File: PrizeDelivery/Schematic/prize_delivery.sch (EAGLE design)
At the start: 22 parts, among them Q1 IRL540

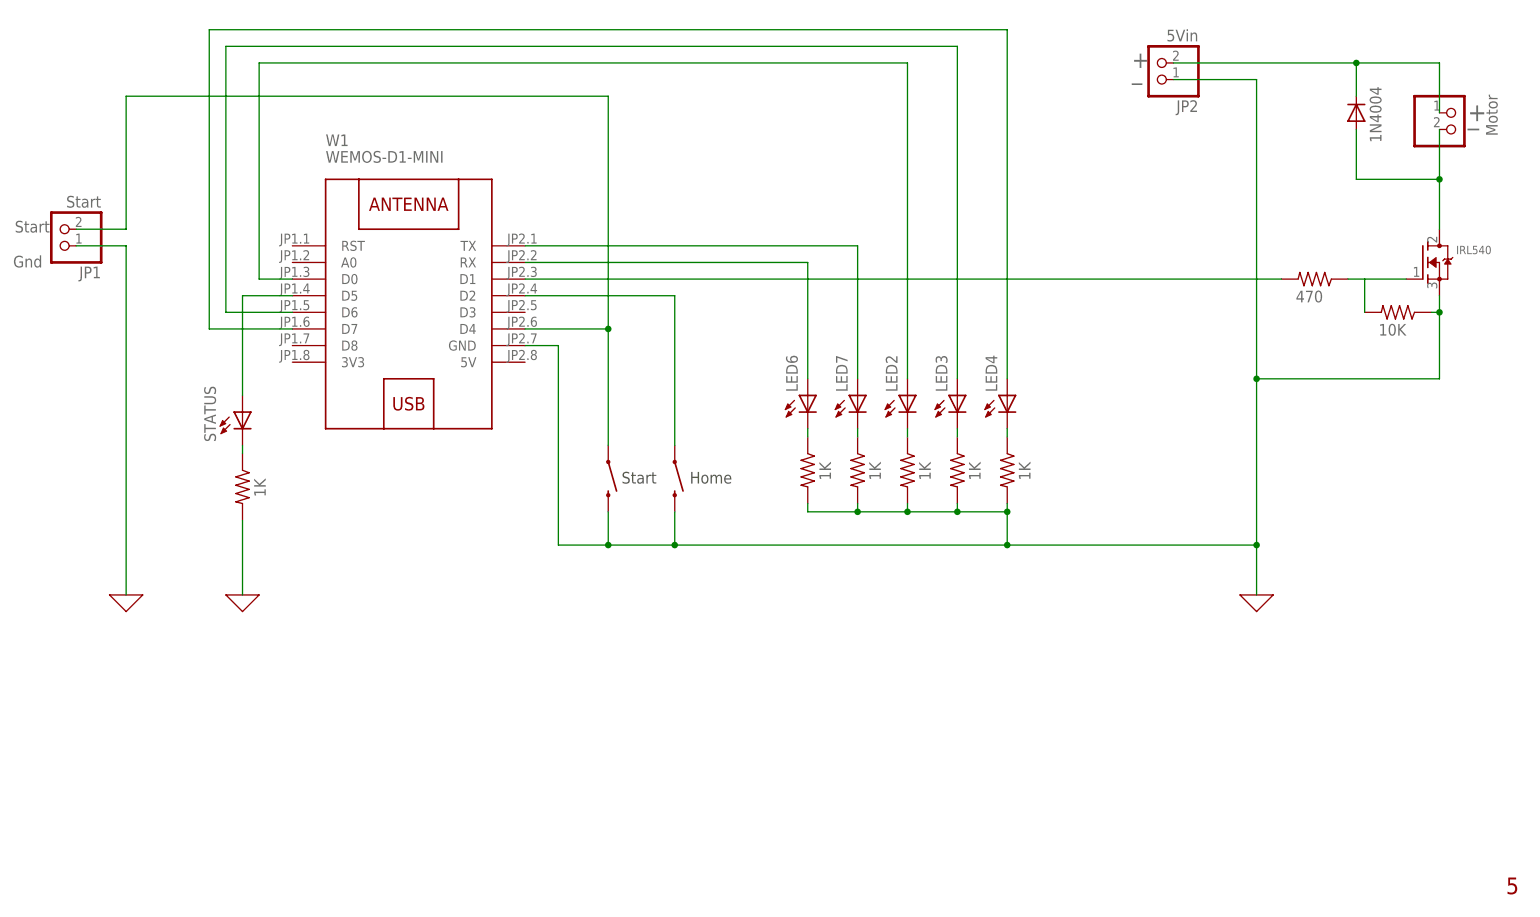
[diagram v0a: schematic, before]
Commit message: Not sure
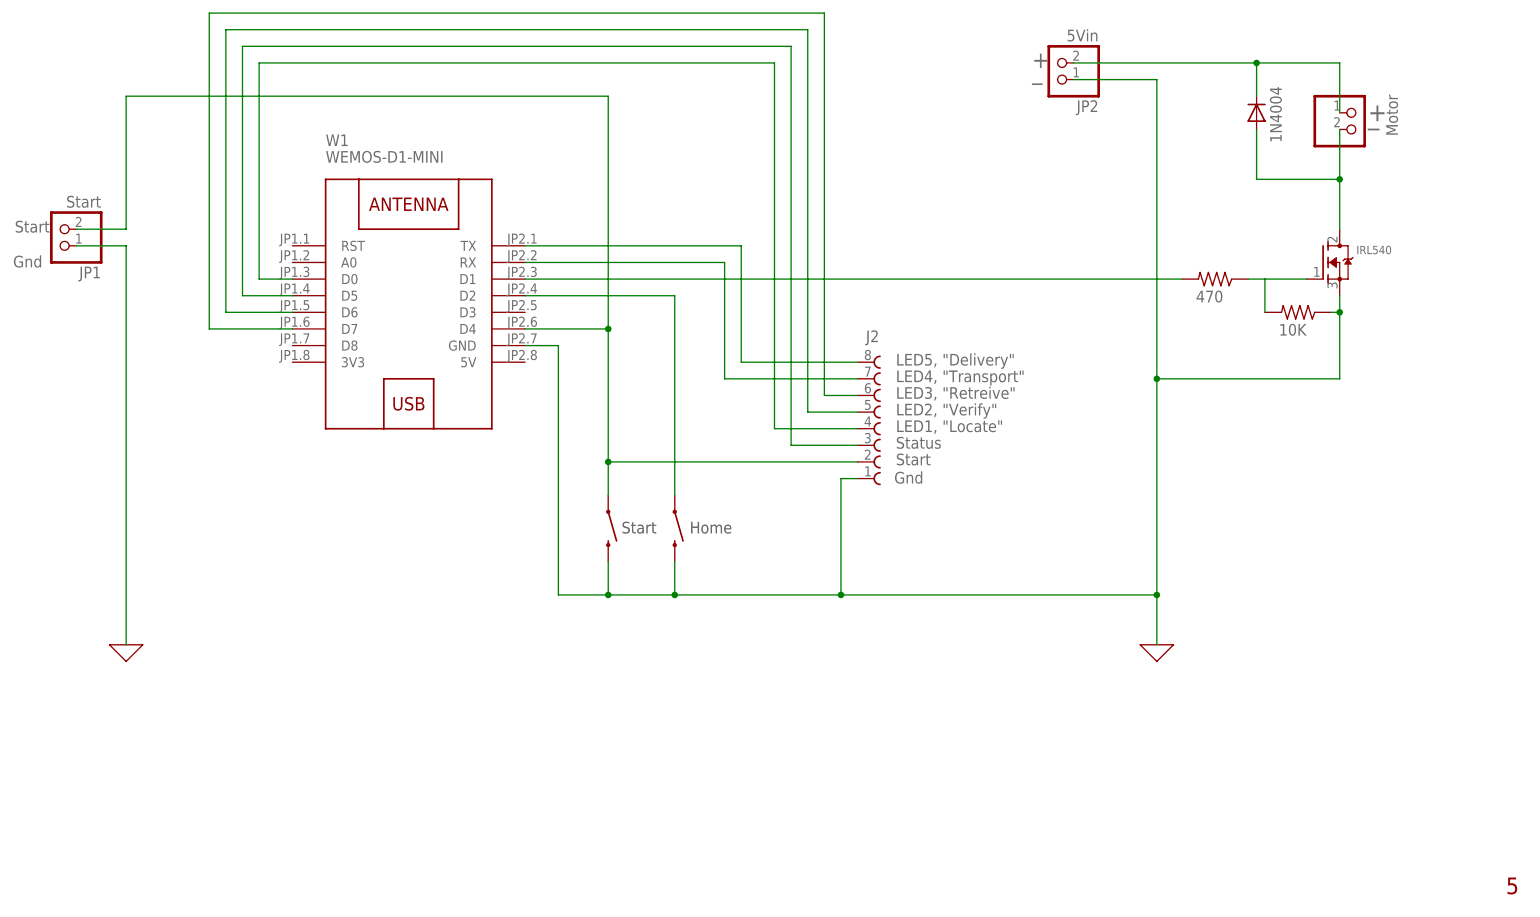
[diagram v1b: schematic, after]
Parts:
- removed LED2, LED3, LED4, LED6, LED7, STATUS: (no value), adafruit:LED5MM
- removed R1, R3, R5, R6, R8, R9: 1K, adafruit:R-US_0207/10
- added J2: (no value), Wurth_Elektronik_Electromechanic_Terminal_Blocks_Connectors_rev19b:691136710008
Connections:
- removed net N$1: LED2.C, R3.1
- removed net N$11: LED6.C, R8.1
- removed net N$12: LED7.C, R9.1
- removed net N$4: LED3.C, R5.1
- removed net N$7: R1.1, STATUS.C
- removed net N$8: LED4.C, R6.1
- net 0: now also J2.1; no longer R1.2, R3.2, R5.2, R6.2, R8.2, R9.2
- net N$15: now also J2.4; no longer LED2.A
- net N$16: now also J2.5; no longer LED3.A
- net N$17: now also J2.6; no longer LED4.A
- net N$18: now also J2.8; no longer LED7.A
- net N$19: now also J2.7; no longer LED6.A
- net N$20: now also J2.3; no longer STATUS.A
- net N$9: now also J2.2
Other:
- note added: "LED1, "Locate""
- note added: "LED2, "Verify""
- note added: "LED3, "Retreive""
- note added: "LED4, "Transport""
- note added: "LED5, "Delivery""
- note added: "Status"
- moved on the sheet: JP2
